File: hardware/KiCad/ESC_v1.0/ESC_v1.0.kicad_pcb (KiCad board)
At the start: 6 copper layers, 156 parts, among them J1 Conn_ARM_SWD_TagConnect_TC203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, J3 USB4105-GF-A, Q1 CSD18540Q5B, Q2 CSD18540Q5B, Q3 CSD18540Q5B, Q4 CSD18540Q5B, Q5 CSD18540Q5B, Q6 CSD18540Q5B, U1 2EDL8024, U2 LM5160A, U3 TPS7B92033, U4 STM32G484CEU6, U5 2EDL8024, U6 2EDL8024, U8 TPD2EUSB30A

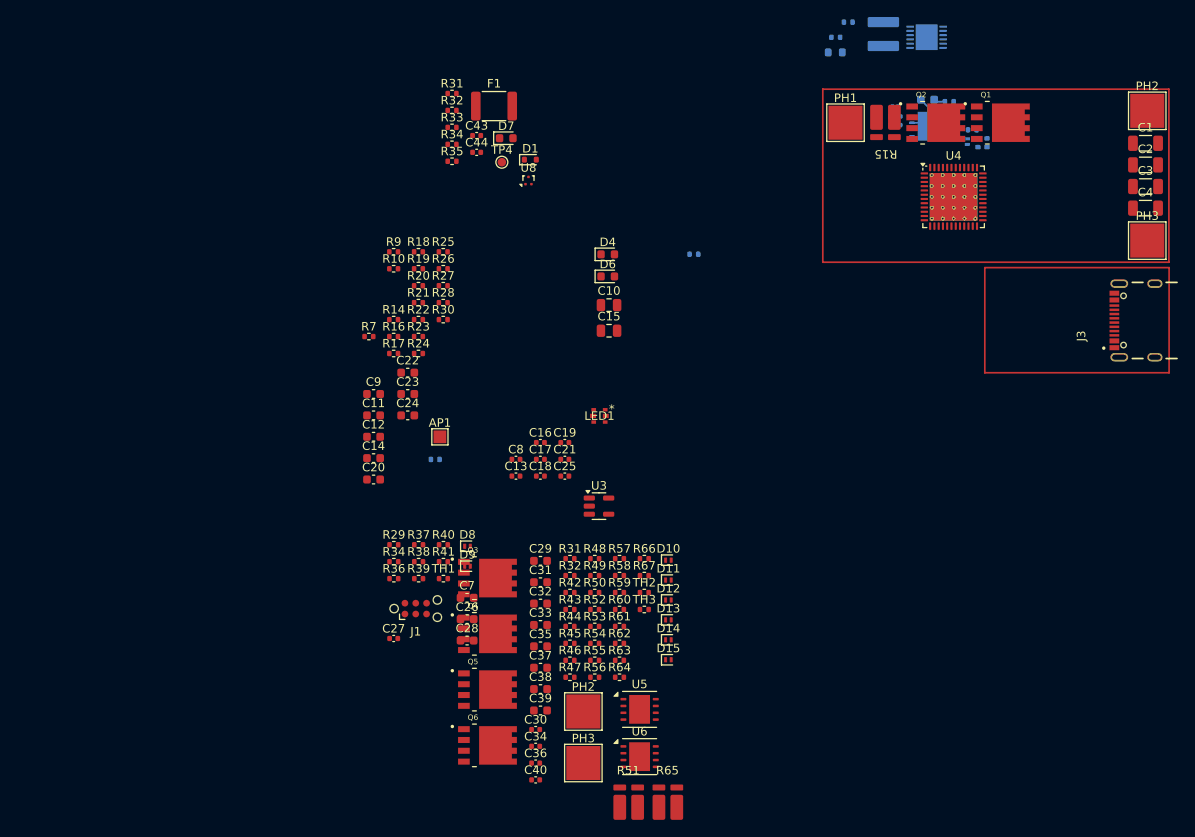
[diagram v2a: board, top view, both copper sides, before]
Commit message: First PCB
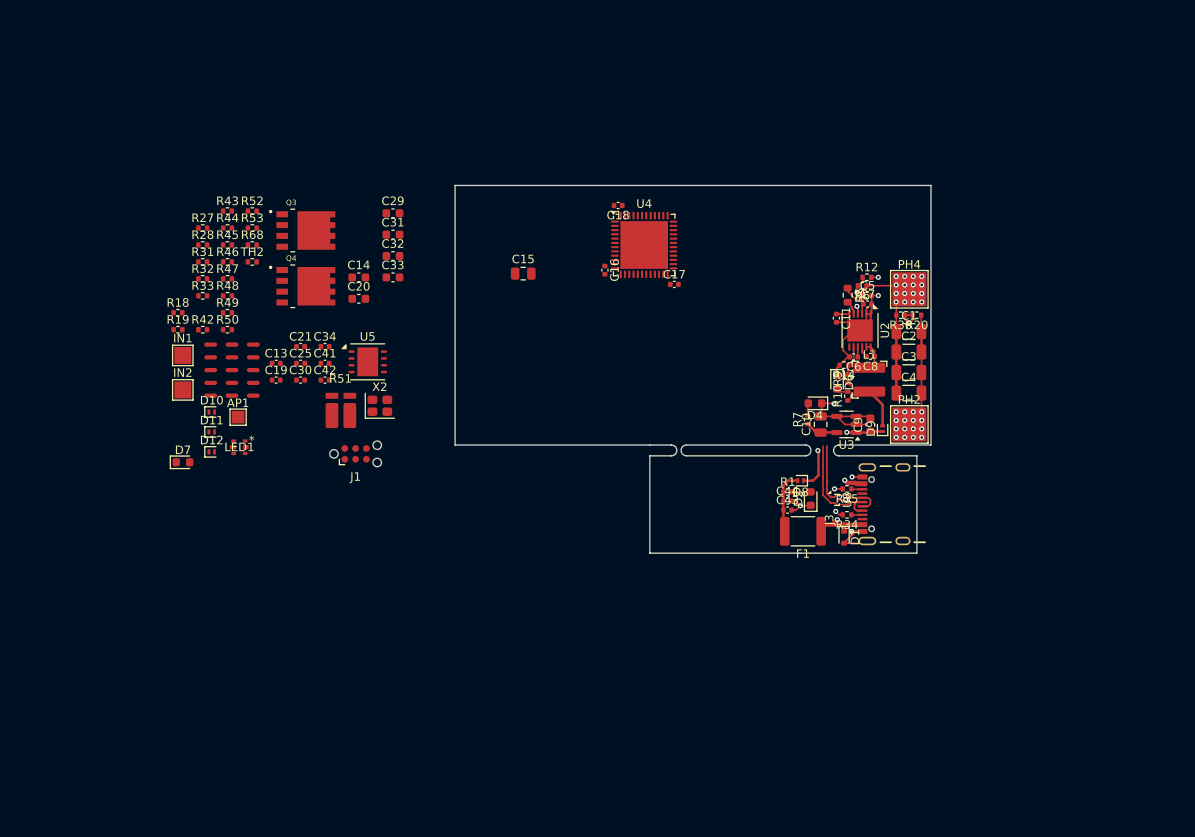
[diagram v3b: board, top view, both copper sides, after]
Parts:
- removed C12, C37: 1u, Capacitor_SMD:C_0603_1608Metric
- removed C22, C23, C24, C26, C28, C35, C38, C39: 100p, Capacitor_SMD:C_0603_1608Metric
- removed C27, C40: 100n, Capacitor_SMD:C_0402_1005Metric
- removed C36: 220n, Capacitor_SMD:C_0402_1005Metric
- removed D13, D14, D15, D3, D5: RB161QS-40T18R, ESC-FootprintLib:Rohm_SMD1006
- removed PH1, PH3 (x2): ~, TestPoint:TestPoint_Pad_4.0x4.0mm
- removed the PH2 at (84.9, 95.9)
- removed the PH2 at (151.1, 25.4)
- removed Q1, Q2, Q5, Q6: CSD18540Q5B, ESC-FootprintLib:TRANS_CSD18540Q5B
- removed R11, R2, R55, R62: 10, Resistor_SMD:R_0402_1005Metric
- removed R13, R16, R17, R30, R4, R40, R41, R58, R59, R64, R67: 10k, Resistor_SMD:R_0402_1005Metric
- removed R15, R65: 0.5m, ESC-FootprintLib:Kelvin Shunt 1216 (3038)
- removed R21, R22, R24, R29, R39, R57, R66: 33, Resistor_SMD:R_0402_1005Metric
- removed R23, R25, R26, R38, R60: 1k, Resistor_SMD:R_0402_1005Metric
- removed R3, R54, R56, R61, R8: 3.3, Resistor_SMD:R_0402_1005Metric
- removed the R31 at (69.5, 23.4)
- removed the R31 at (83.3, 78.0)
- removed the R32 at (83.3, 80.0)
- removed the R32 at (69.5, 25.4)
- removed the R34 at (62.7, 78.3)
- removed the R34 at (69.5, 29.3)
- removed R37, R63: 200k, Resistor_SMD:R_0402_1005Metric
- removed TH1 (x2), TH3: Thermistor_NTC, Resistor_SMD:R_0402_1005Metric
- removed TP4: TestPoint, TestPoint:TestPoint_Pad_D1.0mm
- removed U1, U6: 2EDL8024, ESC-FootprintLib:2EDL8x2x_PG-VDSON-8-4
- added C41: 10p, Capacitor_SMD:C_0402_1005Metric, F.Cu at (54.6, 55.1)
- added C42: 10p, Capacitor_SMD:C_0402_1005Metric, F.Cu at (54.6, 57.0)
- added IN1: ~, TestPoint:TestPoint_Pad_2.0x2.0mm, F.Cu at (37.9, 54.1)
- added IN2: ~, TestPoint:TestPoint_Pad_2.0x2.0mm, F.Cu at (37.9, 58.2)
- added NT1: NetTie_2, NetTie:NetTie-2_SMD_Pad0.5mm, F.Cu at (41.2, 52.8)
- added NT10: NetTie_2, NetTie:NetTie-2_SMD_Pad0.5mm, F.Cu at (43.7, 58.8)
- added NT11: NetTie_2, NetTie:NetTie-2_SMD_Pad0.5mm, F.Cu at (46.2, 52.8)
- added NT12: NetTie_2, NetTie:NetTie-2_SMD_Pad0.5mm, F.Cu at (46.2, 54.3)
- added NT13: NetTie_2, NetTie:NetTie-2_SMD_Pad0.5mm, F.Cu at (46.2, 55.8)
- added NT14: NetTie_2, NetTie:NetTie-2_SMD_Pad0.5mm, F.Cu at (46.2, 57.3)
- added NT15: NetTie_2, NetTie:NetTie-2_SMD_Pad0.5mm, F.Cu at (46.2, 58.8)
- added NT2: NetTie_2, NetTie:NetTie-2_SMD_Pad0.5mm, F.Cu at (41.2, 54.3)
- added NT3: NetTie_2, NetTie:NetTie-2_SMD_Pad0.5mm, F.Cu at (41.2, 55.8)
- added NT4: NetTie_2, NetTie:NetTie-2_SMD_Pad0.5mm, F.Cu at (41.2, 57.3)
- added NT5: NetTie_2, NetTie:NetTie-2_SMD_Pad0.5mm, F.Cu at (41.2, 58.8)
- added NT6: NetTie_2, NetTie:NetTie-2_SMD_Pad0.5mm, F.Cu at (43.7, 52.8)
- added NT7: NetTie_2, NetTie:NetTie-2_SMD_Pad0.5mm, F.Cu at (43.7, 54.3)
- added NT8: NetTie_2, NetTie:NetTie-2_SMD_Pad0.5mm, F.Cu at (43.7, 55.8)
- added NT9: NetTie_2, NetTie:NetTie-2_SMD_Pad0.5mm, F.Cu at (43.7, 57.3)
- added PH2: ~, TestPoint:TestPoint_Pad_4.0x4.0mm, F.Cu at (123.2, 62.2)
- added PH4: ~, TestPoint:TestPoint_Pad_4.0x4.0mm, F.Cu at (123.2, 46.4)
- added R31: 3.3, Resistor_SMD:R_0402_1005Metric, F.Cu at (40.2, 43.1)
- added R32: 10, Resistor_SMD:R_0402_1005Metric, F.Cu at (40.2, 45.1)
- added R34: 5.1k, Resistor_SMD:R_0402_1005Metric, F.Cu at (115.9, 72.8)
- added R68: 0R, Resistor_SMD:R_0402_1005Metric, F.Cu at (46.0, 41.2)
- added X2: 16MHz, Crystal:Crystal_SMD_2520-4Pin_2.5x2.0mm, F.Cu at (61.0, 60.0)
- C11: footprint Capacitor_SMD:C_0603_1608Metric -> Capacitor_SMD:C_0402_1005Metric
- C5: footprint Capacitor_SMD:C_0603_1608Metric -> Capacitor_SMD:C_0402_1005Metric; moved to F.Cu
- C6: value 220n -> 1u; moved to F.Cu
- C7: value 100p -> 1u; footprint Capacitor_SMD:C_0603_1608Metric -> Capacitor_SMD:C_0402_1005Metric
- D2: value RB161QS-40T18R -> KT-0603W; footprint ESC-FootprintLib:Rohm_SMD1006 -> LED_SMD:LED_0603_1608Metric; moved to F.Cu
- L1, R12, R5, R6: moved to F.Cu
- R1: value 3.3 -> 1k; moved to F.Cu
- R20: value 200k -> 10k
- U2: footprint Package_SON:WSON-12-1EP_4x4mm_P0.5mm_EP2.6x3mm -> ESC-FootprintLib:WSON-12-1EP_4x4mm_P0.5mm_EP2.6x3mm; moved to F.Cu
- U4: footprint Package_DFN_QFN:QFN-48-1EP_7x7mm_P0.5mm_EP5.6x5.6mm_ThermalVias -> ESC-FootprintLib:QFN-48-1EP_7x7mm_P0.5mm_EP5.6x5.6mm
- moved R36 67.1 mm to (122.2, 49.4), turned to 180 degrees
- moved F1 61.7 mm to (110.7, 74.8), turned to 180 degrees
- moved R43 61.7 mm to (43.1, 37.2)
- moved R45 61.7 mm to (43.1, 41.2)
- moved R46 61.7 mm to (43.1, 43.1)
- moved R47 61.7 mm to (43.1, 45.1)
- moved R44 61.7 mm to (43.1, 39.2)
- moved R52 61.7 mm to (46.0, 37.2)
- moved R53 61.7 mm to (46.0, 39.2)
- moved R35 60.3 mm to (115.9, 69.8), turned to 180 degrees
- moved TH2 60.2 mm to (46.0, 43.1)
- moved R20 58.6 mm to (124.1, 49.4), turned to 180 degrees
- moved C9 58.5 mm to (118.6, 62.3), turned to 90 degrees
- moved C7 58.3 mm to (118.3, 48.1)
- moved D1 57.6 mm to (115.5, 75.5), turned to -90 degrees
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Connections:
- net +10.5VNoise renamed /SW
- net Net-(D8-K) renamed /VIN
- net TSENS3 renamed /TSENS1
- AP1 pad 1: Net-(AP1-Pad1) -> PWM2
- C1 pad 1: VM -> VBAT
- C13 pad 1: +3V3A -> +3V3
- C13 pad 2: AGND -> GND
- C14 pad 1: +3V3A -> +3V3
- C14 pad 2: AGND -> GND
- C19 pad 1: +3V3REF -> +3V3
- C19 pad 2: AGND -> GND
- C2 pad 1: VM -> VBAT
- C20 pad 1: +3V3REF -> +3V3
- C20 pad 2: AGND -> GND
- C21 pad 1: +3.3V -> +3V3
- C29 pad 1: +VSENS3 -> /+VSENS1
- C3 pad 1: VM -> VBAT
- C30 pad 2: PH2 -> PH1
- C31 pad 1: +10V -> VBUCK
- C32 pad 1: PWM2N -> PWM1N
- C33 pad 1: PWM2 -> PWM1
- C4 pad 1: VM -> VBAT
- C5 pad 1: +10V -> VBAT
- C6 pad 1: /HB1 -> Net-(U2-VCC)
- C6 pad 2: PH1 -> GND
- C7 pad 1: PWM1 -> VBAT
- D1 pad 1: Net-(D1-K) -> /VBUS
- D2 pad 1: /HB1 -> GND
- D9 pad 2: +10.5V -> VBUCK
- F1 pad 1: Net-(D1-K) -> /VBUS
- J1 pad 1: +3.3V -> +3V3
- L1 pad 2: +10.5V -> VBUCK
- LED1 pad 2: +3.3V -> +3V3
- LED1 pad 4: +3.3V -> +3V3
- LED1 pad 6: +3.3V -> +3V3
- Q3 pad 1: VM -> VBAT
- Q3 pad 3: PH2 -> PH1
- Q4 pad 1: PH2 -> PH1
- Q4 pad 3: +ISENS2 -> /+ISENS1
- R1 pad 1: /HO -> +5V
- R1 pad 2: Net-(Q1-G) -> Net-(D2-A)
- R10 pad 1: +10.5V -> VBUCK
- R20 pad 1: Net-(AP1-Pad1) -> GND
- R20 pad 2: GND -> /VSENSBAT
- R36 pad 1: VBAT -> /VSENSBAT
- R36 pad 2: VM -> VBAT
- R43 pad 1: +VSENS3 -> /+VSENS1
- R44 pad 2: PH2 -> PH1
- R46 pad 1: -VSENS3 -> GND
- R49 pad 1: PWM2 -> PWM1
- R5 pad 1: VM -> VBAT
- R51 pad 1: +ISENS2 -> /+ISENS1
- R51 pad 2: Net-(NT9-Pad2) -> /-ISENS1
- R6 pad 1: VM -> VBAT
- R9 pad 1: +10.5V -> VBUCK
- TH2 pad 1: +ISENS3 -> /+ISENS1
- U2 pad 3: VM -> VBAT
- U2 pad 7: Net-(U2-FPWM) -> unconnected-(U2-FPWM-Pad7)
- U2 pad 9: Net-(U2-FPWM) -> Net-(U2-VCC)
- U4 pad 15: +ISENS2 -> /+ISENS2
- U4 pad 18: +VSENS1 -> /+VSENS1
- U4 pad 20: +3V3REF -> +3V3
- U4 pad 21: +3V3A -> +3V3
- U4 pad 25: +VSENS2 -> /+VSENS2
- U4 pad 26: +TSENS2 -> /+TSENS2
- U4 pad 27: +ISENS3 -> /+ISENS3
- U4 pad 28: +TSENS3 -> /+TSENS3
- U4 pad 30: +VSENS3 -> /+VSENS3
- U4 pad 38: VBAT -> /VSENSBAT
- U4 pad 5: unconnected-(U4-PF0-OSC_IN-Pad5) -> Net-(U4-PF0-OSC_IN)
- U4 pad 6: unconnected-(U4-PF1-OSC_OUT-Pad6) -> Net-(U4-PF1-OSC_OUT)
- U4 pad 8: +TSENS1 -> /+TSENS1
- U4 pad 9: +ISENS1 -> /+ISENS1
- U5 pad 1: +10V -> VBUCK
- U5 pad 4: PH2 -> PH1
- U5 pad 5: PWM2 -> PWM1
- U5 pad 6: PWM2N -> PWM1N
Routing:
- net GND: track 5.53 -> 69.7 mm, vias 0 -> 25
- net VBAT: track 0.00 -> 25.6 mm, vias 0 -> 16
- net /VIN: track 0.00 -> 14.3 mm, vias 0 -> 2
- net /VBUS: track 0.00 -> 13.8 mm, vias 0 -> 2
- net USB_D-: track 0.00 -> 13.5 mm
- net USB_D+: track 0.00 -> 12.7 mm
- net VBUCK: track 0.00 -> 10.6 mm
- net +5V: track 0.00 -> 7.37 mm
- net Net-(U2-EN/UVLO): track 0.00 -> 4.63 mm, vias 0 -> 2
- net /HB1: track 4.52 -> 0.00 mm
- net +3V3: track 0.00 -> 3.85 mm
- net Net-(U2-FB): track 0.00 -> 3.51 mm
- net /SW: track 0.00 -> 3.38 mm
- net /VSENSBAT: track 0.00 -> 3.20 mm, vias 0 -> 1
- net +10V: track 3.07 -> 0.00 mm
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- added copper zone on In1.Cu, net GND
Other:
- board outline added: 55.9 x 43.2 mm
